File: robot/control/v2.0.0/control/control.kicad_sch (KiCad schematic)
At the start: 14 parts, among them J1 EC3-M, J9 10033527-N3112MLF

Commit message: WIP
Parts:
- J1: footprint AT-Connectors:XT60-M_TH_WireMount -> AT-Connectors:EC3-M_TH_WireMount
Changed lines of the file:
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@@
     (comment 1 "W. Stuckey & R. Osawa")
   )
+  (bus_alias "RADIO" (members "RADIO.~{RST}" "RADIO.BOOT0" "RADIO.TX" "RADIO.RX" "RADIO.CTS" "RADIO.RTS" "RADIO.~{DET}"))
+  (bus_alias "EXTLOGIC" (members "EXTLOGIC.TX" "EXTLOGIC.RX" "EXTLOGIC.CK" "EXTLOGIC.NSS" "EXTLOGIC.~{DET}"))
   (bus_alias "SDMMC" (members "SDMMC.CMD" "SDMMC.D0" "SDMMC.D1" "SDMMC.D2" "SDMMC.D3" "SDMMC.CK"))
+  (bus_alias "FLOW" (members "FLOW.TX" "FLOW.RX" "FLOW.BOOT0" "FLOW.~{RST}" "FLOW.~{DET}"))
   (bus_alias "KICKER" (members "KICKER.~{DET}" "KICKER.PWRON" "KICKER.TX" "KICKER.RX" "KICKER.BOOT0" "KICKER.~{RST}"))
-  (bus_alias "FLOW" (members "FLOW.TX" "FLOW.RX" "FLOW.BOOT0" "FLOW.~{RST}" "FLOW.~{DET}"))
-  (bus_alias "EXTLOGIC" (members "EXTLOGIC.TX" "EXTLOGIC.RX" "EXTLOGIC.CK" "EXTLOGIC.NSS" "EXTLOGIC.~{DET}"))
-  (bus_alias "RADIO" (members "RADIO.~{RST}" "RADIO.BOOT0" "RADIO.TX" "RADIO.RX" "RADIO.CTS" "RADIO.RTS" "RADIO.~{DET}"))
   (bus_alias "IMU" (members "IMU.~{SS}1" "IMU.~{SS}2" "IMU.~{SS}3" "IMU.MOSI" "IMU.MISO" "IMU.SCK" "IMU.INT1" "IMU.INT2" "IMU.~{DET}" "IMU.~{SS}0"))
   (junction (at 40.64 24.13) (diameter 0) (color 0 0 0 0)
@@
       (effects (font (size 1.27 1.27)))
     )
-    (property "Footprint" "AT-Connectors:XT60-M_TH_WireMount" (at 33.02 26.67 0)
-      (effects (font (size 1.27 1.27)) hide)
-    )
+    (property "Footprint" "AT-Connectors:EC3-M_TH_WireMount" (at 33.02 26.67 0)
+      (effects (font (size 1.27 1.27)) hide)
+    )

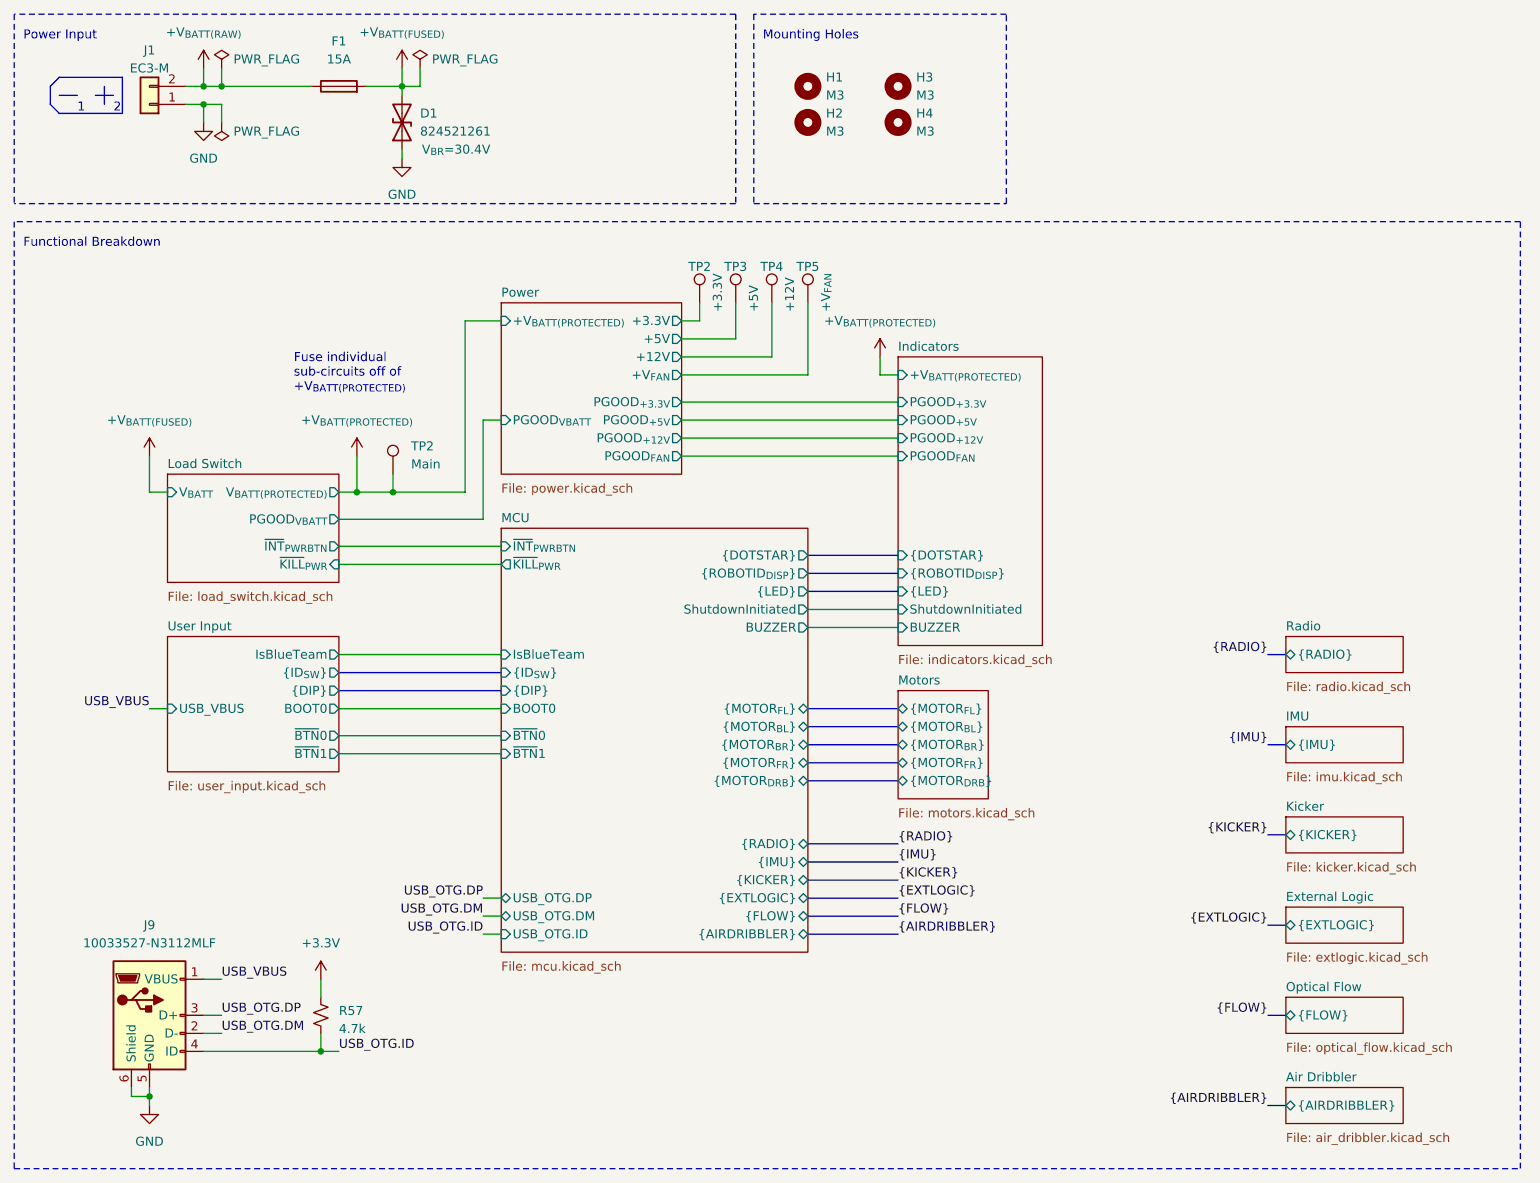
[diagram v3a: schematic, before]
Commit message: WIP
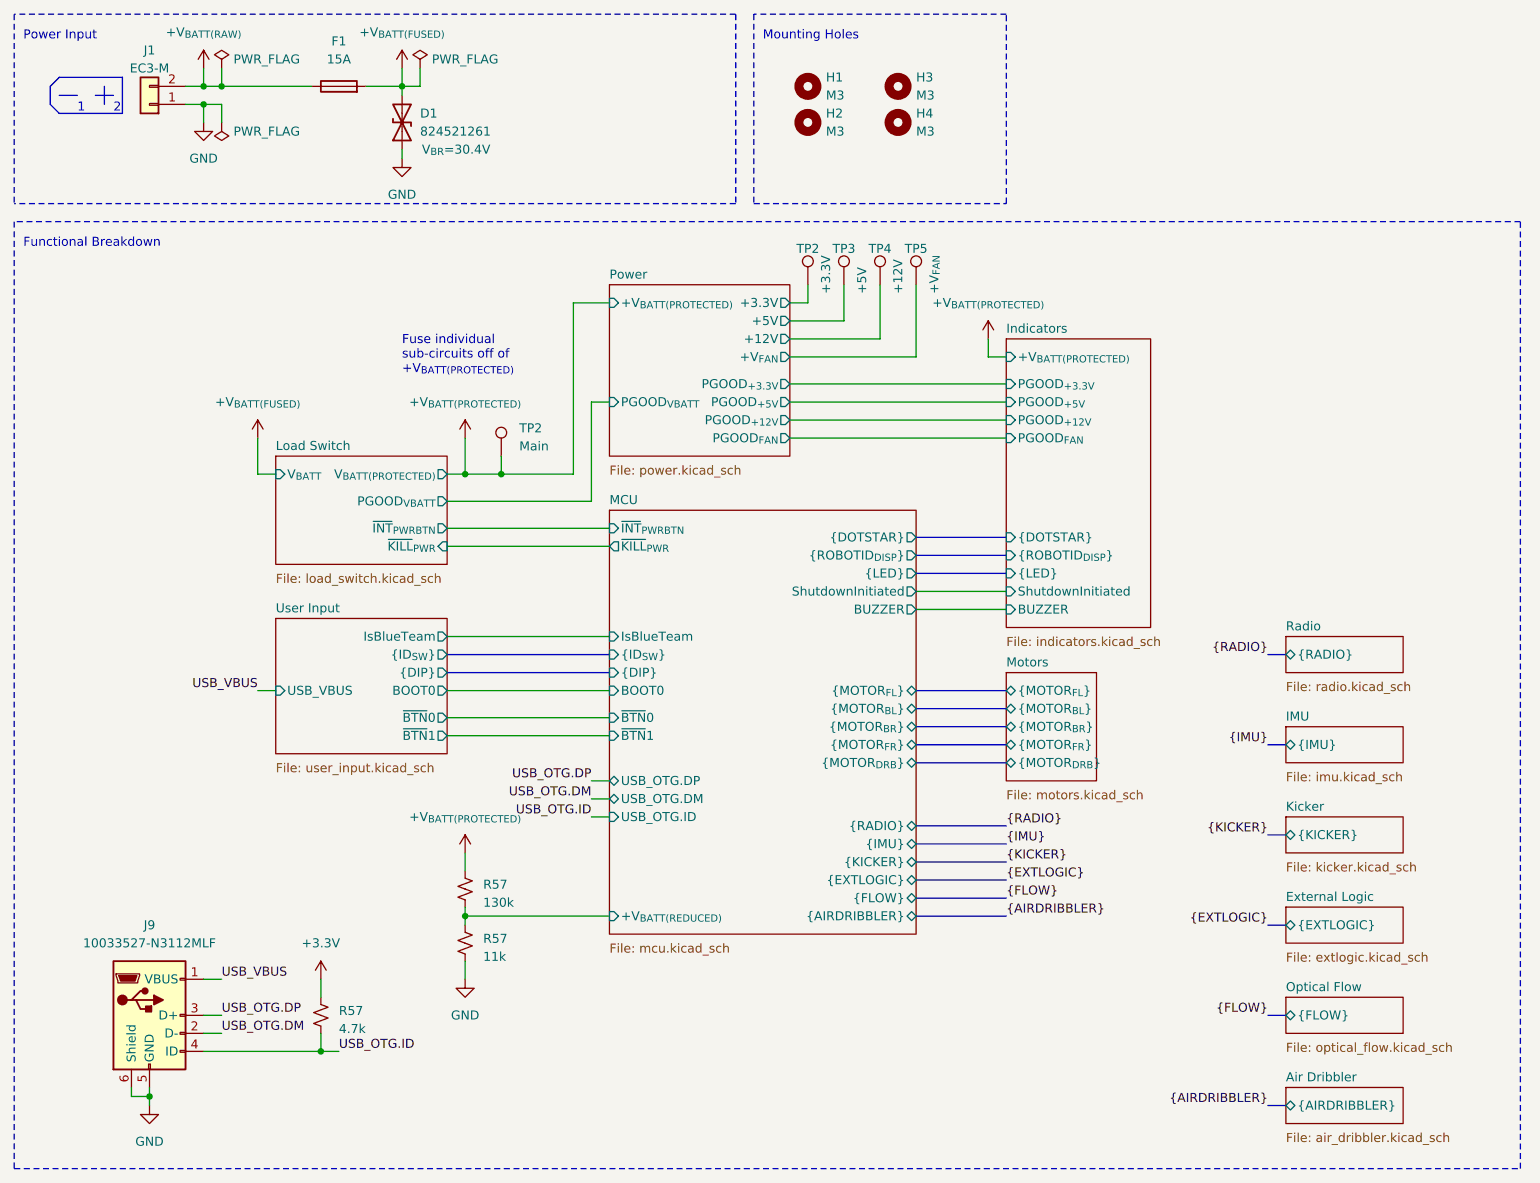
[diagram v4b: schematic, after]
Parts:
- added R57: 130k, Resistor_SMD:R_0402_1005Metric, symbol Device:R_Small_US
- added R57: 11k, Resistor_SMD:R_0402_1005Metric, symbol Device:R_Small_US
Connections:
- net +V_{BATT(PROTECTED)}: now also R57.1
- net GND: now also R57.2
- new net MCU/+V_{BATT(REDUCED)}: R57.1, R57.2
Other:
- sheet MCU ports: added +V_{BATT(REDUCED)}; removed none
- moved on the sheet: TP2, TP3, TP4, TP5
